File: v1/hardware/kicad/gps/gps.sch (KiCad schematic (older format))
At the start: 1 part, among them U1 ublox_SAM-M8Q

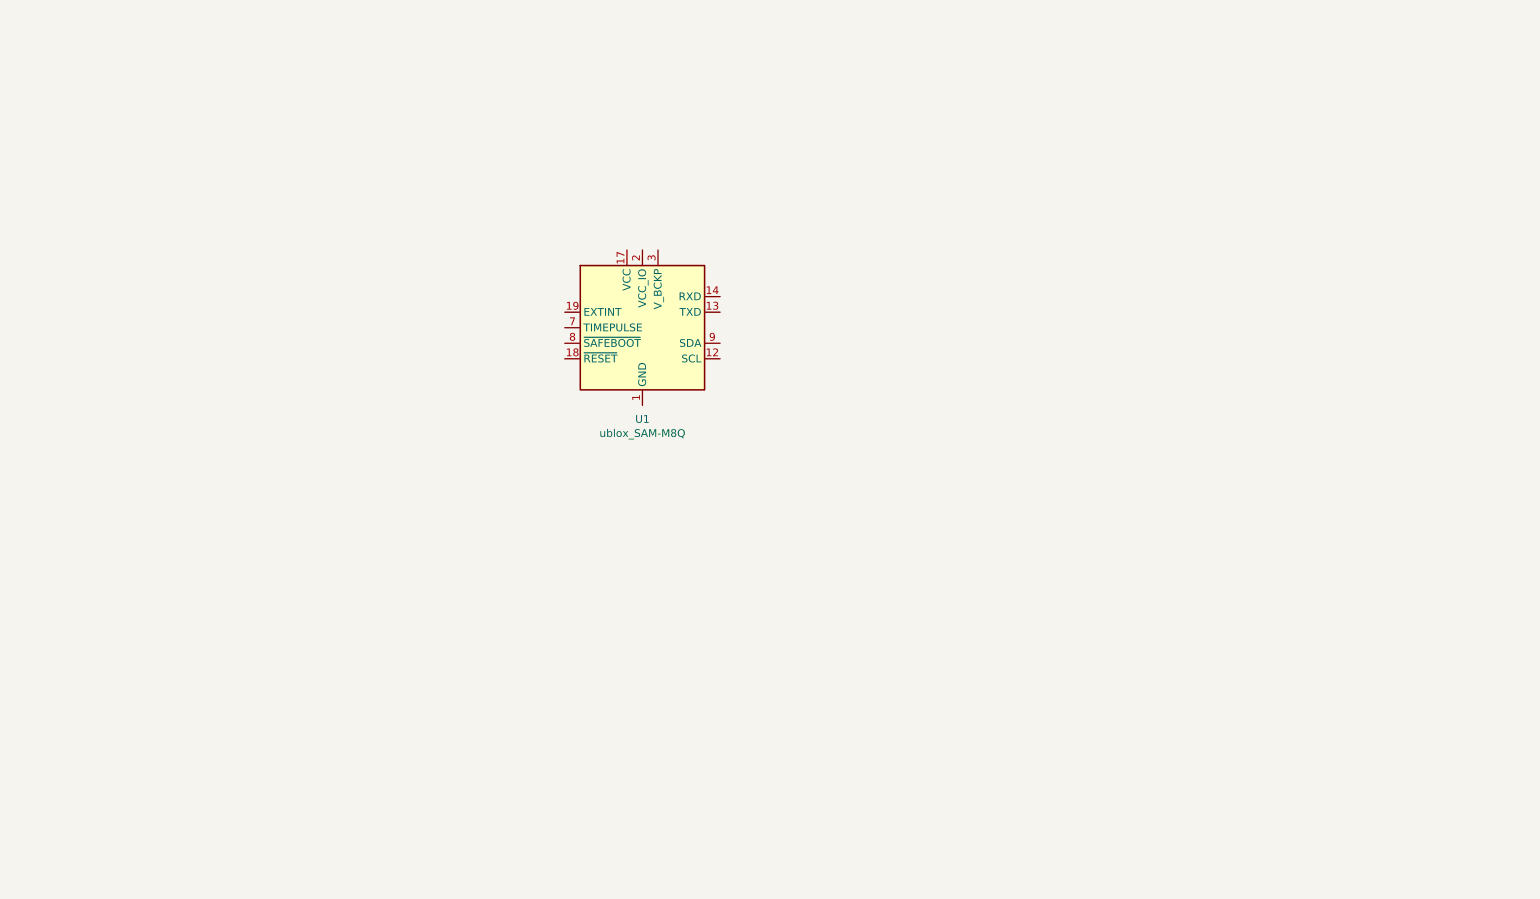
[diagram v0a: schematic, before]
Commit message: update
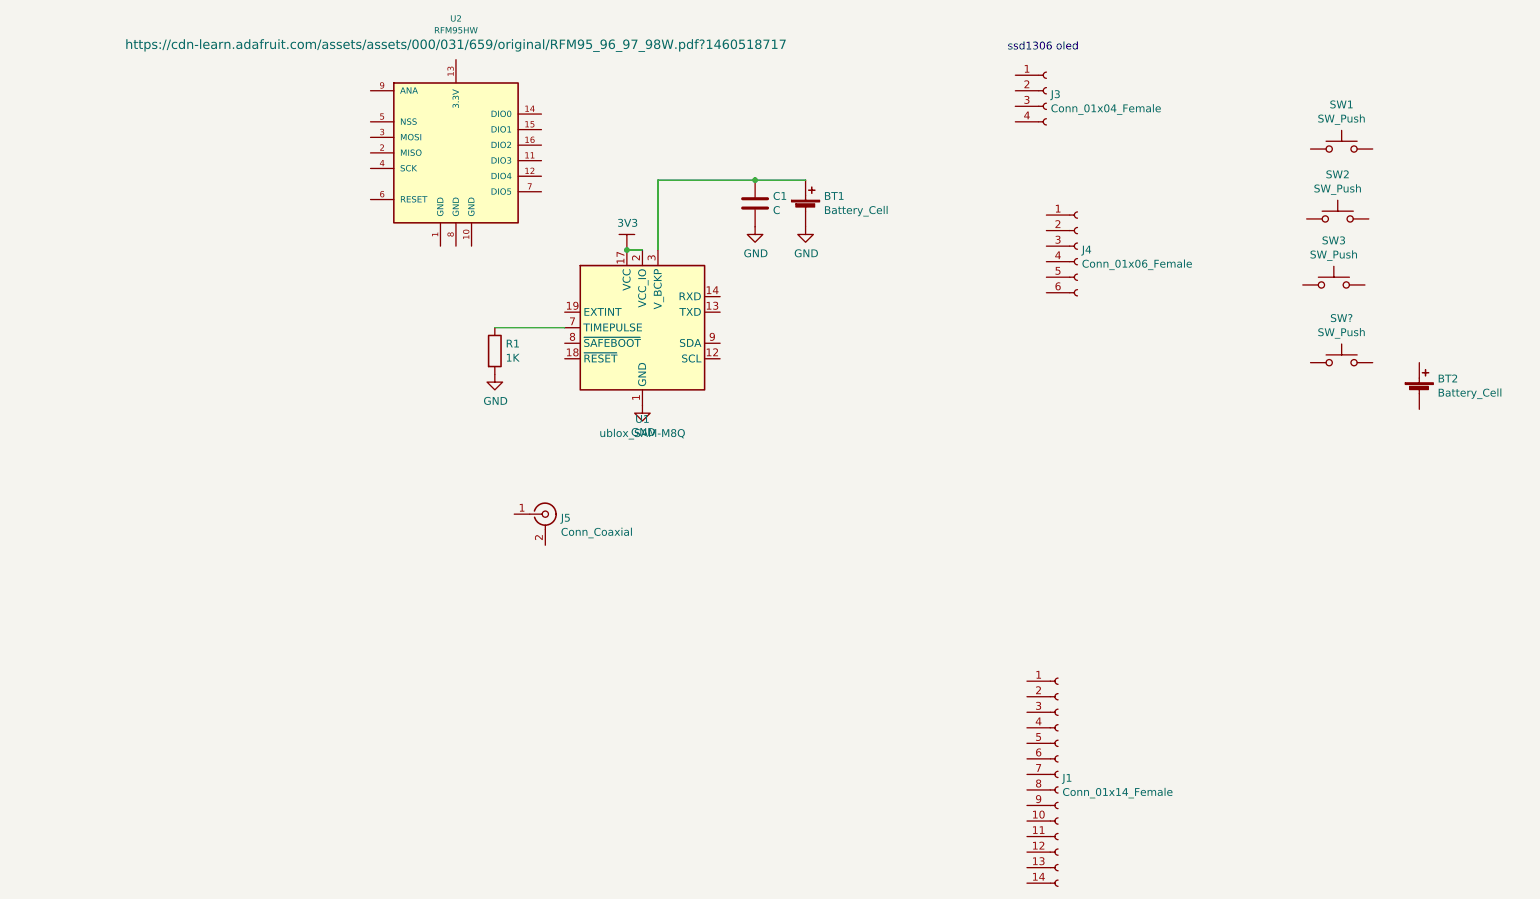
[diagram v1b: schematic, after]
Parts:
- added BT1: Battery_Cell, Battery:BatteryHolder_Keystone_1058_1x2032, symbol Device:Battery_Cell
- added BT2: Battery_Cell, Battery:BatteryHolder_Keystone_1042_1x18650, symbol Device:Battery_Cell
- added C1: C, symbol Device:C
- added J1: Conn_01x14_Female, Connector_PinSocket_2.54mm:PinSocket_1x14_P2.54mm_Vertical, symbol Connector:Conn_01x14_Female
- added J3: Conn_01x04_Female, Connector_PinSocket_2.54mm:PinSocket_1x04_P2.54mm_Vertical, symbol Connector:Conn_01x04_Female
- added J4: Conn_01x06_Female, Connector_PinSocket_2.54mm:PinSocket_1x06_P2.54mm_Vertical, symbol Connector:Conn_01x06_Female
- added J5: Conn_Coaxial, Connector_Coaxial:SMA_Molex_73251-1153_EdgeMount_Horizontal, symbol Connector:Conn_Coaxial
- added R1: 1K, symbol Device:R
- added SW1, SW2, SW3, SW?: SW_Push, Button_Switch_THT:SW_Tactile_SPST_Angled_PTS645Vx58-2LFS, symbol Switch:SW_Push
- added U2: RFM95HW, RF_Module:HOPERF_RFM9XW_SMD, symbol mysensors_radios:RFM95HW
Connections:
- net GND: now reaches U1.1 (GND), U1.10 (GND), U1.11 (GND), U1.15 (GND), U1.16 (GND), U1.20 (GND), U1.4 (GND), U1.5 (GND), U1.6 (GND)
- net GND: now also BT1.2 (-), C1.2, R1.2
- net 3V3: now reaches U1.17 (VCC)
- net 3V3: now also U1.2 (VCC_IO)
- net at U1.3 (V_BCKP): now also BT1.1 (+), C1.1
- net at U1.7 (TIMEPULSE): now also R1.1
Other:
- note added: "ssd1306 oled"
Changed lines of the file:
@@
+	1    0    0    -1
+$EndComp
+$Comp
+L power:GND #PWR0101
+U 1 1 615C8D4D
+P 2950 3275
+F 0 "#PWR0101" H 2950 3025 50  0001 C CNN
+F 1 "GND" H 2955 3102 50  0000 C CNN
+F 2 "" H 2950 3275 50  0001 C CNN
+F 3 "" H 2950 3275 50  0001 C CNN
+	1    2950 3275
+	1    0    0    -1
+$EndComp
+$Comp
+L RocketScreamKicadLibrary:3V3 #PWR0102
+U 1 1 615C945F
+P 2850 2275
+F 0 "#PWR0102" H 2850 2125 50  0001 C CNN
+F 1 "3V3" H 2855 2448 50  0000 C CNN
+F 2 "" H 2850 2275 60  0000 C CNN
+F 3 "" H 2850 2275 60  0000 C CNN
+	1    2850 2275
+	1    0    0    -1
+$EndComp
+Wire Wire Line
+	2450 2775 2000 2775
+$Comp
+L Device:R R1
+U 1 1 615C9F6F
+P 2000 2925
+F 0 "R1" H 2070 2971 50  0000 L CNN
+F 1 "1K" H 2070 2880 50  0000 L CNN
+F 2 "" V 1930 2925 50  0001 C CNN
+F 3 "~" H 2000 2925 50  0001 C CNN
+	1    2000 2925
+	1    0    0    -1
+$EndComp
+$Comp
+L power:GND #PWR0103
+U 1 1 615CA4A4
+P 2000 3075
+F 0 "#PWR0103" H 2000 2825 50  0001 C CNN
+F 1 "GND" H 2005 2902 50  0000 C CNN
+F 2 "" H 2000 3075 50  0001 C CNN
+F 3 "" H 2000 3075 50  0001 C CNN
+	1    2000 3075
+	1    0    0    -1
+$EndComp
+Wire Wire Line
+	2950 2275 2850 2275
+Connection ~ 2850 2275
+$Comp
+L Device:Battery_Cell BT1
+U 1 1 615CB1E5
+P 4000 2025
+F 0 "BT1" H 4118 2121 50  0000 L CNN
+F 1 "Battery_Cell" H 4118 2030 50  0000 L CNN
+F 2 "Battery:BatteryHolder_Keystone_1058_1x2032" V 4000 2085 50  0001 C CNN
+F 3 "~" V 4000 2085 50  0001 C CNN
+	1    4000 2025
+	1    0    0    -1
+$EndComp
+Wire Wire Line
+	4000 1825 3675 1825
+Wire Wire Line
+	3050 1825 3050 2275
+$Comp
+L Device:C C1
+U 1 1 615CD5CD
+P 3675 1975
+F 0 "C1" H 3790 2021 50  0000 L CNN
+F 1 "C" H 3790 1930 50  0000 L CNN
+F 2 "" H 3713 1825 50  0001 C CNN
+F 3 "~" H 3675 1975 50  0001 C CNN
+	1    3675 1975
+	1    0    0    -1
+$EndComp
+Connection ~ 3675 1825
+Wire Wire Line
+	3675 1825 3050 1825
+$Comp
+L power:GND #PWR0104
+U 1 1 615CDEE4
+P 3675 2125
+F 0 "#PWR0104" H 3675 1875 50  0001 C CNN
+F 1 "GND" H 3680 1952 50  0000 C CNN
+F 2 "" H 3675 2125 50  0001 C CNN
+F 3 "" H 3675 2125 50  0001 C CNN
+	1    3675 2125
+	1    0    0    -1
+$EndComp
+$Comp
+L power:GND #PWR0105
+U 1 1 615CE1BE
+P 4000 2125
+F 0 "#PWR0105" H 4000 1875 50  0001 C CNN
+F 1 "GND" H 4005 1952 50  0000 C CNN
+F 2 "" H 4000 2125 50  0001 C CNN
+F 3 "" H 4000 2125 50  0001 C CNN
+	1    4000 2125
+	1    0    0    -1
+$EndComp
+$Comp
+L mysensors_radios:RFM95HW U2
+U 1 1 615D66DF
+P 1750 1400
+F 0 "U2" H 1750 2014 40  0000 C CNN
+F 1 "RFM95HW" H 1750 1938 40  0000 C CNN
+F 2 "RF_Module:HOPERF_RFM9XW_SMD" H 1750 1400 30  0001 C CIN
+F 3 "https://cdn-learn.adafruit.com/assets/assets/000/031/659/original/RFM95_96_97_98W.pdf?1460518717" H 1750 1847 60  0000 C CNN
+	1    1750 1400
+	1    0    0    -1
+$EndComp
+$Comp
+L Connector:Conn_01x04_Female J3
+U 1 1 615DA9EE
+P 5550 1250
+F 0 "J3" H 5578 1226 50  0000 L CNN
+F 1 "Conn_01x04_Female" H 5578 1135 50  0000 L CNN
+F 2 "Connector_PinSocket_2.54mm:PinSocket_1x04_P2.54mm_Vertical" H 5550 1250 50  0001 C CNN
+F 3 "~" H 5550 1250 50  0001 C CNN
+	1    5550 1250
+	1    0    0    -1
+$EndComp
+Text Notes 5300 1000 0    50   ~ 0
+ssd1306 oled
+$Comp
+L Connector:Conn_01x06_Female J4
+U 1 1 615E1B8F
+P 5750 2250
+F 0 "J4" H 5778 2226 50  0000 L CNN
+F 1 "Conn_01x06_Female" H 5778 2135 50  0000 L CNN
+F 2 "Connector_PinSocket_2.54mm:PinSocket_1x06_P2.54mm_Vertical" H 5750 2250 50  0001 C CNN
+F 3 "~" H 5750 2250 50  0001 C CNN
+	1    5750 2250
+	1    0    0    -1
+$EndComp
+$Comp
+L Switch:SW_Push SW1
+U 1 1 615E9717
+P 7450 1625
+F 0 "SW1" H 7450 1910 50  0000 C CNN
+F 1 "SW_Push" H 7450 1819 50  0000 C CNN
+F 2 "Button_Switch_THT:SW_Tactile_SPST_Angled_PTS645Vx58-2LFS" H 7450 1825 50  0001 C CNN
+F 3 "~" H 7450 1825 50  0001 C CNN
+	1    7450 1625
+	1    0    0    -1
+$EndComp
+$Comp
+L Switch:SW_Push SW2
+U 1 1 615EB759
+P 7425 2075
+F 0 "SW2" H 7425 2360 50  0000 C CNN
+F 1 "SW_Push" H 7425 2269 50  0000 C CNN
+F 2 "Button_Switch_THT:SW_Tactile_SPST_Angled_PTS645Vx58-2LFS" H 7425 2275 50  0001 C CNN
+F 3 "~" H 7425 2275 50  0001 C CNN
+	1    7425 2075
+	1    0    0    -1
+$EndComp
+$Comp
+L Connector:Conn_Coaxial J5
+U 1 1 615EF508
+P 2325 3975
+F 0 "J5" H 2425 3950 50  0000 L CNN
+F 1 "Conn_Coaxial" H 2425 3859 50  0000 L CNN
+F 2 "Connector_Coaxial:SMA_Molex_73251-1153_EdgeMount_Horizontal" H 2325 3975 50  0001 C CNN
+F 3 " ~" H 2325 3975 50  0001 C CNN
+	1    2325 3975
+	1    0    0    -1
+$EndComp
+$Comp
+L Device:Battery_Cell BT2
+U 1 1 6160C21F
+P 7950 3200
+F 0 "BT2" H 8068 3296 50  0000 L CNN
+F 1 "Battery_Cell" H 8068 3205 50  0000 L CNN
+F 2 "Battery:BatteryHolder_Keystone_1042_1x18650" V 7950 3260 50  0001 C CNN
+F 3 "~" V 7950 3260 50  0001 C CNN
+	1    7950 3200
+	1    0    0    -1
+$EndComp
+$Comp
+L Connector:Conn_01x14_Female J1
+U 1 1 61641A77
+P 5625 5650
+F 0 "J1" H 5653 5626 50  0000 L CNN
+F 1 "Conn_01x14_Female" H 5653 5535 50  0000 L CNN
+F 2 "Connector_PinSocket_2.54mm:PinSocket_1x14_P2.54mm_Vertical" H 5625 5650 50  0001 C CNN
+F 3 "~" H 5625 5650 50  0001 C CNN
+	1    5625 5650
+	1    0    0    -1
+$EndComp
+$Comp
+L Switch:SW_Push SW3
+U 1 1 6164981D
+P 7400 2500
+F 0 "SW3" H 7400 2785 50  0000 C CNN
+F 1 "SW_Push" H 7400 2694 50  0000 C CNN
+F 2 "Button_Switch_THT:SW_Tactile_SPST_Angled_PTS645Vx58-2LFS" H 7400 2700 50  0001 C CNN
+F 3 "~" H 7400 2700 50  0001 C CNN
+	1    7400 2500
+	1    0    0    -1
+$EndComp
+$Comp
+L Switch:SW_Push SW?
+U 1 1 6164AA87
+P 7450 3000
+F 0 "SW?" H 7450 3285 50  0000 C CNN
+F 1 "SW_Push" H 7450 3194 50  0000 C CNN
+F 2 "Button_Switch_THT:SW_Tactile_SPST_Angled_PTS645Vx58-2LFS" H 7450 3200 50  0001 C CNN
+F 3 "~" H 7450 3200 50  0001 C CNN
+	1    7450 3000
 	1    0    0    -1
 $EndComp
